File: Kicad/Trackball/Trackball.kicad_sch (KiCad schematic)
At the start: 67 parts, among them J1 Battery, J10 Female, J11 Conn_01x04_Female, J12 Conn_01x04_Female, J13 Female, J14 Conn_01x04_Female, J15 Conn_01x04_Female, J17 Conn_01x04_Female, J18 Conn_01x03_Pin, J19 Conn_01x03_Pin, J2 Male, J20 Conn_01x03_Socket, J21 Conn_01x03_Socket, J3 Male, J4 Conn_01x04_Male, J5 Conn_01x04_Male, J7 Conn_01x04_Male, J8 Conn_01x04_Male, J9 Conn_01x04_Male, SW1 SW_SPDT, SW2 SW_SPDT, SW3 SW_SPDT, U1 ProMicro, U3 TCR2EF19, U4 PMW3610

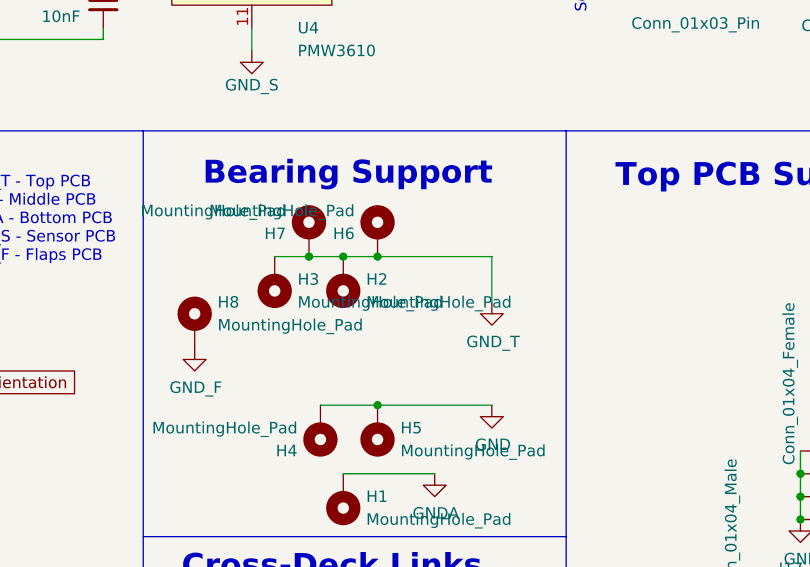
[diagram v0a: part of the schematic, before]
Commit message: B5: Rev.1 changes.
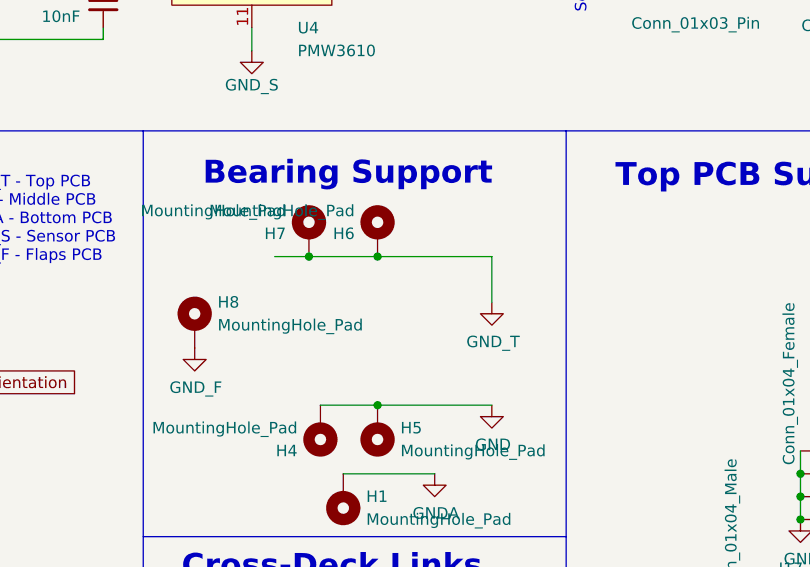
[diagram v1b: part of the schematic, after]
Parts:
- removed H2, H3: MountingHole_Pad, MountingHole:MountingHole_2.5mm_Pad, symbol Mechanical:MountingHole_Pad
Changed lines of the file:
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@@
 	)
 	(junction
-		(at 208.28 91.44)
-		(diameter 0)
-		(color 0 0 0 0)
-	)
-	(junction
 		(at 267.97 138.43)
 		(diameter 0)
@@
 	(wire
 		(pts
-			(xy 204.47 91.44) (xy 208.28 91.44)
-		)
-		(stroke
-			(width 0)
-			(type default)
-		)
-	)
-	(wire
-		(pts
 			(xy 87.63 149.86) (xy 87.63 147.32)
 		)
@@
 	(wire
 		(pts
-			(xy 208.28 91.44) (xy 212.09 91.44)
+			(xy 204.47 91.44) (xy 212.09 91.44)
 		)
 		(stroke
@@
 	)
 	(symbol
-		(lib_id "Mechanical:MountingHole_Pad")
-		(at 208.28 93.98 180)
-		(unit 1)
-		(exclude_from_sim no)
-		(in_bom no)
-		(on_board yes)
-		(dnp no)
-		(fields_autoplaced yes)
-		(property "Reference" "H2"
-			(at 210.82 93.9799 0)
-			(effects
-				(font
-					(size 1.27 1.27)
-				)
-				(justify right)
-			)
-		)
-		(property "Value" "MountingHole_Pad"
-			(at 210.82 96.5199 0)
-			(effects
-				(font
-					(size 1.27 1.27)
-				)
-				(justify right)
-			)
-		)
-		(property "Footprint" "MountingHole:MountingHole_2.5mm_Pad"
-			(at 208.28 93.98 0)
-			(effects
-				(font
-					(size 1.27 1.27)
-				)
-				(hide yes)
-			)
-		)
-		(property "Datasheet" "~"
-			(at 208.28 93.98 0)
-			(effects
-				(font
-					(size 1.27 1.27)
-				)
-				(hide yes)
-			)
-		)
-		(property "Description" "Mounting Hole with connection"
-			(at 208.28 93.98 0)
-			(effects
-				(font
-					(size 1.27 1.27)
-				)
-				(hide yes)
-			)
-		)
-		(pin "1"
-		)
-		(instances
-			(project "Trackball"
-				(path "/8cc78baa-4975-41f7-8a0a-10f41c28d40d"
-					(reference "H2")
-					(unit 1)
-				)
-			)
-		)
-	)
-	(symbol
 		(lib_id "Device:C_Small")
 		(at 165.1 63.5 0)
@@
 					(unit 1)
 				)
-			)
-		)
-	)
-	(symbol
-		(lib_id "Mechanical:MountingHole_Pad")
-		(at 200.66 93.98 180)
-		(unit 1)
-		(exclude_from_sim no)
-		(in_bom no)
-		(on_board yes)
-		(dnp no)
-		(fields_autoplaced yes)
-		(property "Reference" "H3"
-			(at 203.2 93.9799 0)
-			(effects
-				(font
-					(size 1.27 1.27)
-				)
-				(justify right)
-			)
-		)
-		(property "Value" "MountingHole_Pad"
-			(at 203.2 96.5199 0)
-			(effects
-				(font
-					(size 1.27 1.27)
-				)
-				(justify right)
-			)
-		)
-		(property "Footprint" "MountingHole:MountingHole_2.5mm_Pad"
-			(at 200.66 93.98 0)
-			(effects
-				(font
-					(size 1.27 1.27)
-				)
-				(hide yes)
-			)
-		)
-		(property "Datasheet" "~"
-			(at 200.66 93.98 0)
-			(effects
-				(font
-					(size 1.27 1.27)
-				)
-				(hide yes)
-			)
-		)
-		(property "Description" "Mounting Hole with connection"
-			(at 200.66 93.98 0)
-			(effects
-				(font
-					(size 1.27 1.27)
-				)
-				(hide yes)
-			)
-		)
-		(pin "1"
-		)
-		(instances
-			(project "Trackball"
-				(path "/8cc78baa-4975-41f7-8a0a-10f41c28d40d"
-					(reference "H3")
-					(unit 1)
-				)
